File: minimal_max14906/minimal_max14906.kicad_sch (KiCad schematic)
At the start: 83 parts, among them J1 CLP-114-02-G-D-BE, J10 TBP02R2-381-02BE, J11 TBP02R2-381-02BE, J2 CLP-102-02-G-D-BE, J3 CLP-102-02-G-D-BE, J4 CLP-102-02-G-D-BE, J5 CLP-102-02-G-D-BE, J6 CLP-102-02-G-D-BE, J7 CLP-102-02-G-D-BE, J8 TBP02R2-381-02BE, J9 TBP02R2-381-02BE, Q1 -60.0 V, Q2 -60.0 V, Q3 -60.0 V, Q4 -60.0 V, U1 MAX14906ATM+

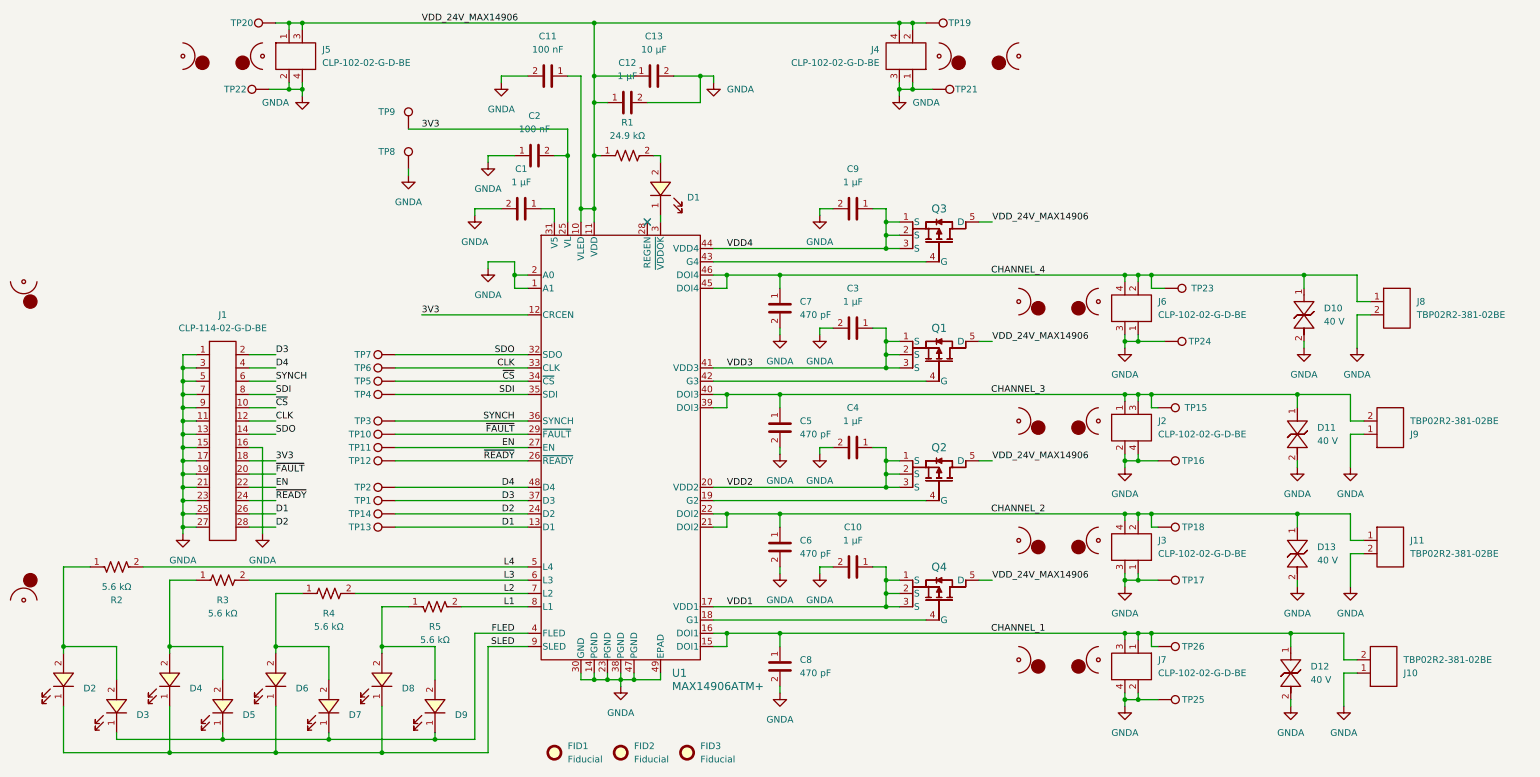
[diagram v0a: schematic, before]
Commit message: Switch to KiCad 9
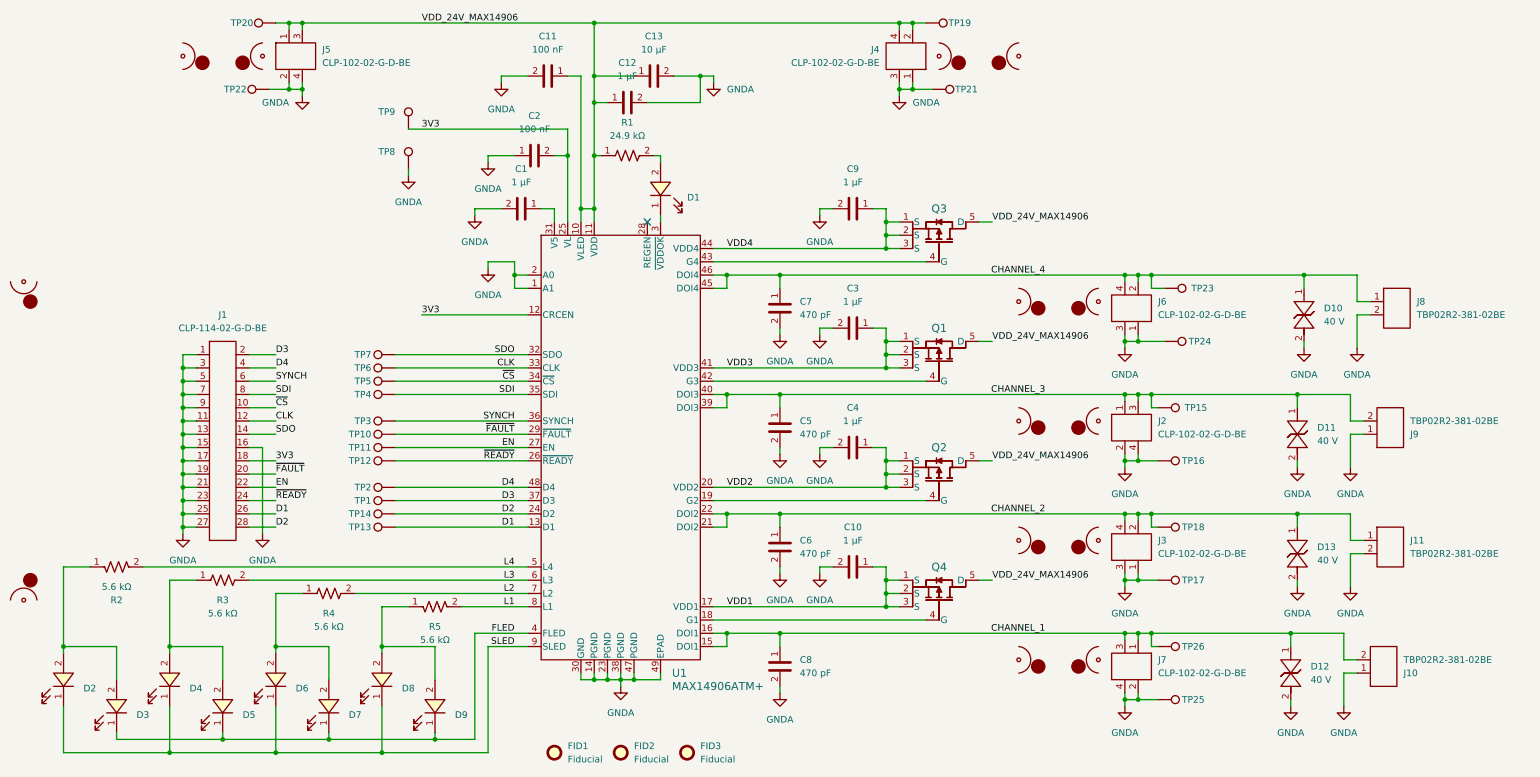
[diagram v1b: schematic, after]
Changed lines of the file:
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@@
 (kicad_sch
-	(version 20231120)
+	(version 20250114)
 	(generator "eeschema")
-	(generator_version "8.0")
+	(generator_version "9.0")
 	(paper "A3")
 	(junction
@@
 		)
 	)
+	(embedded_fonts no)
 )
